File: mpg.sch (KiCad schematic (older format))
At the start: 47 parts, among them J1 DB25_Male_MountingHoles, J2 Conn_01x04_Male, J3 Conn_01x03_Male, J4 Conn_01x02_Male, J5 RJ45_Shielded, Q1 BC847, Q2 BC847, Q3 BC847, Q4 BC847, Q5 BC847, SW1 SW_Push, U1 LD2981ABU33TR, U2 STM32G431K6Tx, U3 SN65HVD230, U4 ESDCAN24-2BLY, Y1 8MHz

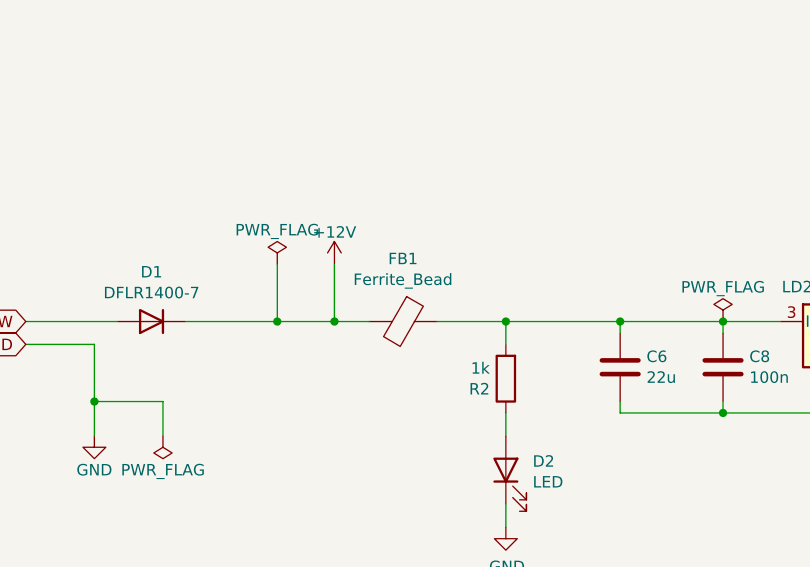
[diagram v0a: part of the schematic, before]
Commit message: Final layout.
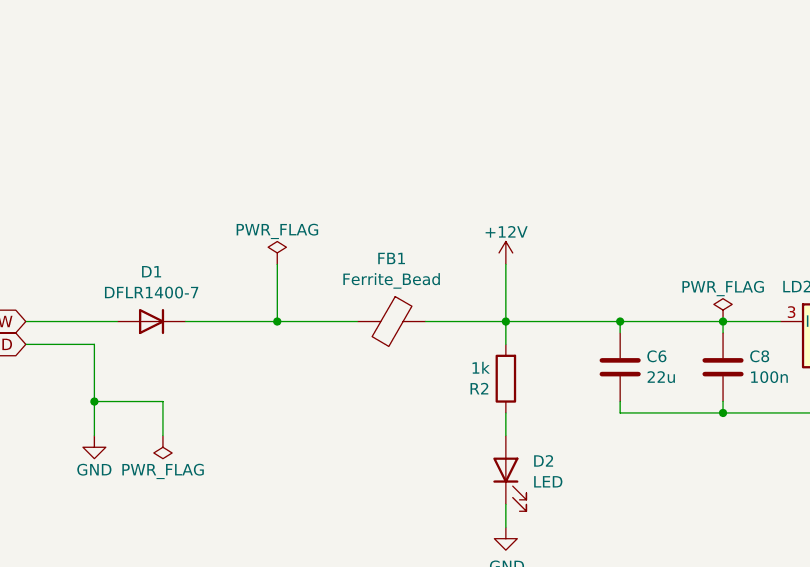
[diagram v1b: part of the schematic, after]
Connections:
- net +12V: now also C6.1, C8.1, FB1.1, R2.2, U1.3 (IN); no longer D1.1 (K), FB1.2
- new net: D1.1 (K), FB1.2
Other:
- moved on the sheet: FB1
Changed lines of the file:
@@
 $EndComp
 Wire Wire Line
-	5450 9700 5750 9700
+	5400 9700 5750 9700
 $Comp
 L Device:Ferrite_Bead FB?
 U 1 1 6017CB65
-P 5300 9700
+P 5250 9700
 AR Path="/5F2EFD7F/6017CB65" Ref="FB?"  Part="1"
 AR Path="/6017CB65" Ref="FB1"  Part="1"
@@
 AR Path="/61500A32/6017CB65" Ref="FB?"  Part="1"
 AR Path="/60152FAB/6017CB65" Ref="FB?"  Part="1"
-F 0 "FB1" V 5026 9700 50  0000 C CNN
-F 1 "Ferrite_Bead" V 5117 9700 50  0000 C CNN
-F 2 "Inductor_SMD:L_0603_1608Metric" V 5230 9700 50  0001 C CNN
-F 3 "~" H 5300 9700 50  0001 C CNN
-	1    5300 9700
+F 0 "FB1" V 4976 9700 50  0000 C CNN
+F 1 "Ferrite_Bead" V 5067 9700 50  0000 C CNN
+F 2 "Inductor_SMD:L_0603_1608Metric" V 5180 9700 50  0001 C CNN
+F 3 "~" H 5250 9700 50  0001 C CNN
+	1    5250 9700
 	0    1    1    0
 $EndComp
@@
 L power:+12V #PWR?
 U 1 1 6017CC57
-P 5000 9450
+P 5750 9450
 AR Path="/5F2EFD7F/6017CC57" Ref="#PWR?"  Part="1"
 AR Path="/6017CC57" Ref="#PWR010"  Part="1"
@@
 AR Path="/61500A32/6017CC57" Ref="#PWR?"  Part="1"
 AR Path="/60152FAB/6017CC57" Ref="#PWR?"  Part="1"
-F 0 "#PWR010" H 5000 9300 50  0001 C CNN
-F 1 "+12V" H 5000 9590 50  0000 C CNN
-F 2 "" H 5000 9450 50  0001 C CNN
-F 3 "" H 5000 9450 50  0001 C CNN
-	1    5000 9450
+F 0 "#PWR010" H 5750 9300 50  0001 C CNN
+F 1 "+12V" H 5750 9590 50  0000 C CNN
+F 2 "" H 5750 9450 50  0001 C CNN
+F 3 "" H 5750 9450 50  0001 C CNN
+	1    5750 9450
 	1    0    0    -1
 $EndComp
@@
 Wire Wire Line
 	4750 9700 4750 9450
-Wire Wire Line
-	5000 9450 5000 9700
 $Comp
 L power:PWR_FLAG #FLG?
@@
 $EndComp
 Connection ~ 4750 9700
-Connection ~ 5000 9700
-Wire Wire Line
-	5000 9700 4750 9700
 Wire Wire Line
 	5750 10500 5750 10600
@@
 	3900 2400 4000 2400
 Wire Wire Line
-	5000 9700 5150 9700
-Wire Wire Line
 	5750 9800 5750 9700
 Connection ~ 5750 9700
 Wire Wire Line
 	5750 9700 6250 9700
+Wire Wire Line
+	4750 9700 5100 9700
+Wire Wire Line
+	5750 9450 5750 9700
 $EndSCHEMATC
